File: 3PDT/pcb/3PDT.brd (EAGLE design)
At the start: 29.8 x 26.7 mm, 4 parts, among them SW1 3PDT, X1 2510-

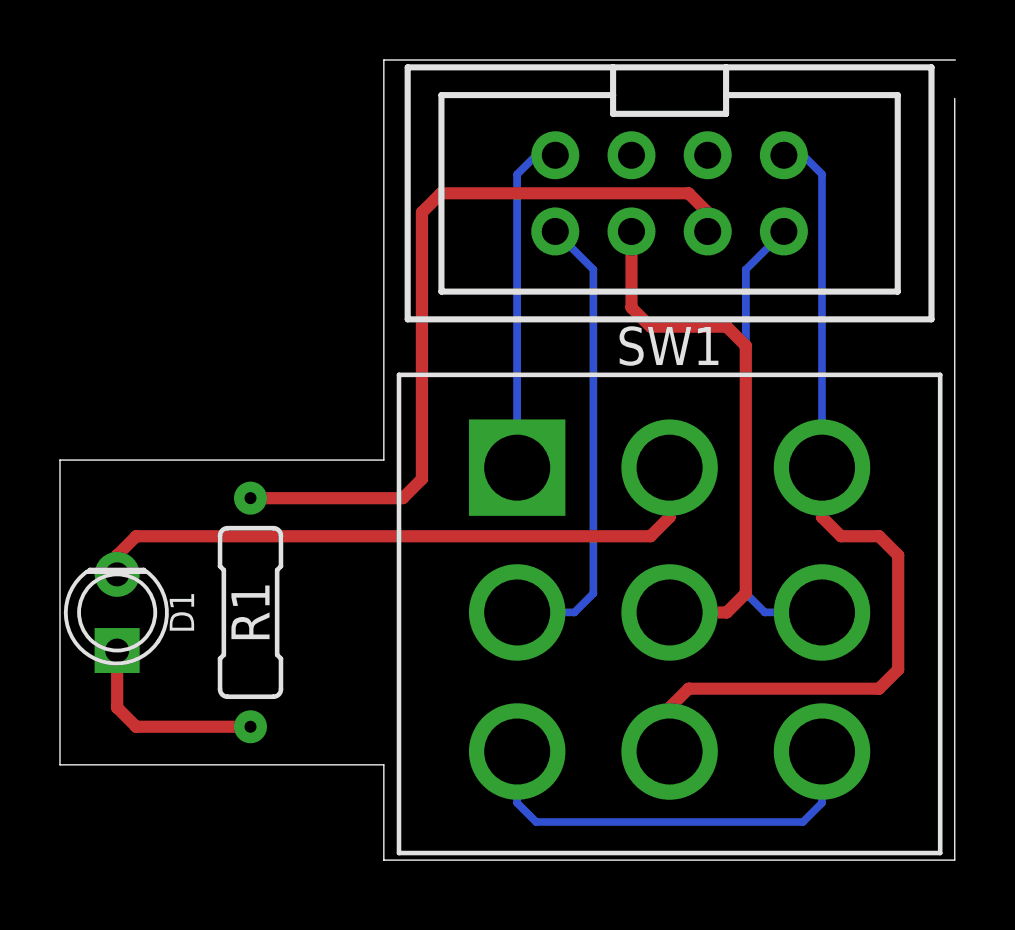
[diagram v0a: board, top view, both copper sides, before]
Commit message: 20170914
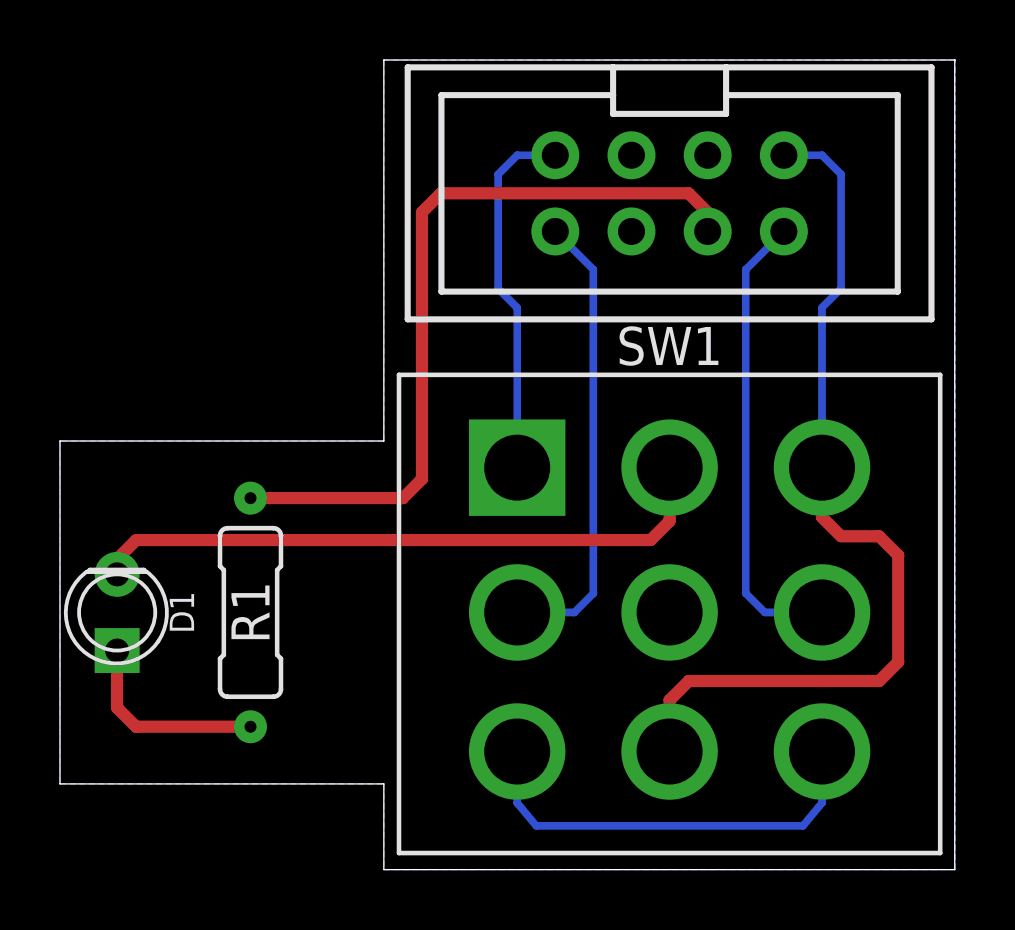
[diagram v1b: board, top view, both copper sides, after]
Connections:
- net N$6 renamed GND
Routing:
- net GND: track 17.9 -> 0.00 mm
- net N$3: track 29.4 -> 30.3 mm
- net N$5: track 11.3 -> 12.2 mm
- added copper zone on layer 16, net GND
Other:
- board size 29.8 x 26.7 mm -> 29.8 x 27 mm
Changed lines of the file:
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@@
 <board>
 <plain>
-<wire x1="10.795" y1="0" x2="29.825" y2="0" width="0" layer="20"/>
-<wire x1="29.825" y1="0" x2="29.825" y2="25.3875" width="0" layer="20"/>
-<wire x1="0" y1="13.335" x2="0" y2="3.175" width="0" layer="20"/>
-<wire x1="10.795" y1="26.67" x2="10.795" y2="13.335" width="0" layer="20"/>
-<wire x1="10.795" y1="13.335" x2="0" y2="13.335" width="0" layer="20"/>
+<wire x1="10.795" y1="-0.3175" x2="29.825" y2="-0.3175" width="0" layer="20"/>
+<wire x1="29.825" y1="-0.3175" x2="29.8243625" y2="26.6702" width="0" layer="20"/>
+<wire x1="0" y1="13.97" x2="0" y2="2.54" width="0" layer="20"/>
+<wire x1="10.795" y1="26.67" x2="10.795" y2="13.97" width="0" layer="20"/>
+<wire x1="10.795" y1="13.97" x2="0" y2="13.97" width="0" layer="20"/>
 <wire x1="10.795" y1="26.67" x2="29.845" y2="26.67" width="0" layer="20"/>
-<wire x1="0" y1="3.175" x2="10.795" y2="3.175" width="0" layer="20"/>
-<wire x1="10.795" y1="3.175" x2="10.795" y2="0" width="0" layer="20"/>
+<wire x1="0" y1="2.54" x2="10.795" y2="2.54" width="0" layer="20"/>
+<wire x1="10.795" y1="2.54" x2="10.795" y2="-0.3175" width="0" layer="20"/>
 </plain>
 <attributes>
@@
 <contactref element="SW1" pad="C3"/>
 <contactref element="SW1" pad="A3"/>
-<wire x1="15.24" y1="1.905" x2="15.875" y2="1.27" width="0.254" layer="16"/>
-<wire x1="15.875" y1="1.27" x2="24.765" y2="1.27" width="0.254" layer="16"/>
-<wire x1="24.765" y1="1.27" x2="25.4" y2="1.905" width="0.254" layer="16"/>
+<wire x1="15.24" y1="1.905" x2="15.875" y2="1.143" width="0.254" layer="16"/>
+<wire x1="15.875" y1="1.143" x2="24.765" y2="1.143" width="0.254" layer="16"/>
+<wire x1="24.765" y1="1.143" x2="25.4" y2="1.905" width="0.254" layer="16"/>
 <wire x1="15.24" y1="3.6195" x2="15.24" y2="1.905" width="0.254" layer="16"/>
 <wire x1="25.4" y1="3.6195" x2="25.4" y2="1.905" width="0.254" layer="16"/>
@@
 <contactref element="X1" pad="1"/>
 <contactref element="SW1" pad="B3"/>
-<wire x1="20.955" y1="5.715" x2="27.305" y2="5.715" width="0.4064" layer="1"/>
-<wire x1="27.305" y1="5.715" x2="27.94" y2="6.35" width="0.4064" layer="1"/>
-<wire x1="27.94" y1="6.35" x2="27.94" y2="10.16" width="0.4064" layer="1"/>
+<wire x1="20.955" y1="5.969" x2="27.305" y2="5.969" width="0.4064" layer="1"/>
+<wire x1="27.305" y1="5.969" x2="27.94" y2="6.604" width="0.4064" layer="1"/>
+<wire x1="27.94" y1="6.604" x2="27.94" y2="10.16" width="0.4064" layer="1"/>
 <wire x1="27.94" y1="10.16" x2="27.305" y2="10.795" width="0.4064" layer="1"/>
 <wire x1="27.305" y1="10.795" x2="26.035" y2="10.795" width="0.4064" layer="1"/>
-<wire x1="25.4" y1="22.86" x2="24.765" y2="23.495" width="0.254" layer="16"/>
-<wire x1="24.765" y1="23.495" x2="24.13" y2="23.495" width="0.254" layer="16"/>
-<wire x1="20.955" y1="5.715" x2="20.32" y2="5.08" width="0.4064" layer="1"/>
-<wire x1="20.32" y1="5.08" x2="20.32" y2="3.6195" width="0.4064" layer="1"/>
+<wire x1="20.955" y1="5.969" x2="20.32" y2="5.334" width="0.4064" layer="1"/>
+<wire x1="20.32" y1="5.334" x2="20.32" y2="3.6195" width="0.4064" layer="1"/>
 <wire x1="26.035" y1="10.795" x2="25.4" y2="11.43" width="0.4064" layer="1"/>
 <wire x1="25.4" y1="11.43" x2="25.4" y2="13.081" width="0.4064" layer="1"/>
-<wire x1="25.4" y1="22.86" x2="25.4" y2="13.081" width="0.254" layer="16"/>
+<wire x1="25.4" y1="13.081" x2="25.4" y2="18.415" width="0.254" layer="16"/>
+<wire x1="25.4" y1="18.415" x2="26.035" y2="19.05" width="0.254" layer="16"/>
+<wire x1="26.035" y1="19.05" x2="26.035" y2="22.86" width="0.254" layer="16"/>
+<wire x1="26.035" y1="22.86" x2="25.4" y2="23.495" width="0.254" layer="16"/>
+<wire x1="25.4" y1="23.495" x2="24.13" y2="23.495" width="0.254" layer="16"/>
 </signal>
 <signal name="N$4">
@@
 <contactref element="X1" pad="7"/>
 <contactref element="SW1" pad="A1"/>
-<wire x1="15.24" y1="22.86" x2="15.875" y2="23.495" width="0.254" layer="16"/>
-<wire x1="15.875" y1="23.495" x2="16.51" y2="23.495" width="0.254" layer="16"/>
-<wire x1="15.24" y1="22.86" x2="15.24" y2="13.081" width="0.254" layer="16"/>
-</signal>
-<signal name="N$6">
-<contactref element="X1" pad="6"/>
-<contactref element="SW1" pad="B2"/>
-<wire x1="22.86" y1="8.89" x2="22.86" y2="17.145" width="0.4064" layer="1"/>
-<wire x1="22.86" y1="17.145" x2="22.225" y2="17.78" width="0.4064" layer="1"/>
-<wire x1="22.225" y1="17.78" x2="19.685" y2="17.78" width="0.4064" layer="1"/>
-<wire x1="19.685" y1="17.78" x2="19.05" y2="18.415" width="0.4064" layer="1"/>
-<wire x1="19.05" y1="18.415" x2="19.05" y2="20.955" width="0.4064" layer="1"/>
-<wire x1="20.32" y1="8.255" x2="22.225" y2="8.255" width="0.4064" layer="1"/>
-<wire x1="22.225" y1="8.255" x2="22.86" y2="8.89" width="0.4064" layer="1"/>
+<wire x1="15.24" y1="13.081" x2="15.24" y2="18.415" width="0.254" layer="16"/>
+<wire x1="15.24" y1="18.415" x2="14.605" y2="19.05" width="0.254" layer="16"/>
+<wire x1="14.605" y1="19.05" x2="14.605" y2="22.86" width="0.254" layer="16"/>
+<wire x1="14.605" y1="22.86" x2="15.24" y2="23.495" width="0.254" layer="16"/>
+<wire x1="15.24" y1="23.495" x2="16.51" y2="23.495" width="0.254" layer="16"/>
 </signal>
 <signal name="N$7">
@@
 <contactref element="D1" pad="P$1"/>
 <contactref element="SW1" pad="B1"/>
-<wire x1="1.905" y1="9.525" x2="1.905" y2="10.16" width="0.4064" layer="1"/>
-<wire x1="1.905" y1="10.16" x2="2.54" y2="10.795" width="0.4064" layer="1"/>
-<wire x1="2.54" y1="10.795" x2="19.685" y2="10.795" width="0.4064" layer="1"/>
-<wire x1="19.685" y1="10.795" x2="20.32" y2="11.43" width="0.4064" layer="1"/>
-<wire x1="20.32" y1="11.43" x2="20.32" y2="13.081" width="0.4064" layer="1"/>
+<wire x1="1.905" y1="9.525" x2="1.905" y2="10.033" width="0.4064" layer="1"/>
+<wire x1="1.905" y1="10.033" x2="2.54" y2="10.668" width="0.4064" layer="1"/>
+<wire x1="2.54" y1="10.668" x2="19.685" y2="10.668" width="0.4064" layer="1"/>
+<wire x1="19.685" y1="10.668" x2="20.32" y2="11.303" width="0.4064" layer="1"/>
+<wire x1="20.32" y1="11.303" x2="20.32" y2="13.081" width="0.4064" layer="1"/>
+</signal>
+<signal name="GND">
+<contactref element="X1" pad="6"/>
+<contactref element="SW1" pad="B2"/>
+<polygon width="0.3048" layer="16" isolate="0.2032">
+<vertex x="10.795" y="26.67"/>
+<vertex x="10.795" y="13.97"/>
+<vertex x="0" y="13.97"/>
+<vertex x="0" y="2.54"/>
+<vertex x="10.795" y="2.54"/>
+<vertex x="10.795" y="-0.3175"/>
+<vertex x="29.845" y="-0.3175"/>
+<vertex x="29.845" y="26.67"/>
+</polygon>
 </signal>
 </signals>
